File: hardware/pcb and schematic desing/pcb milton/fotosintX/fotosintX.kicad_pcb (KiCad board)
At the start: 2 copper layers, 46.5 x 74.3 mm, 12 parts, among them J4 TB_1X2, J5 TB_1X2, Q1 2N3904, U1 ESP32_DEVKITC, U2 L7805

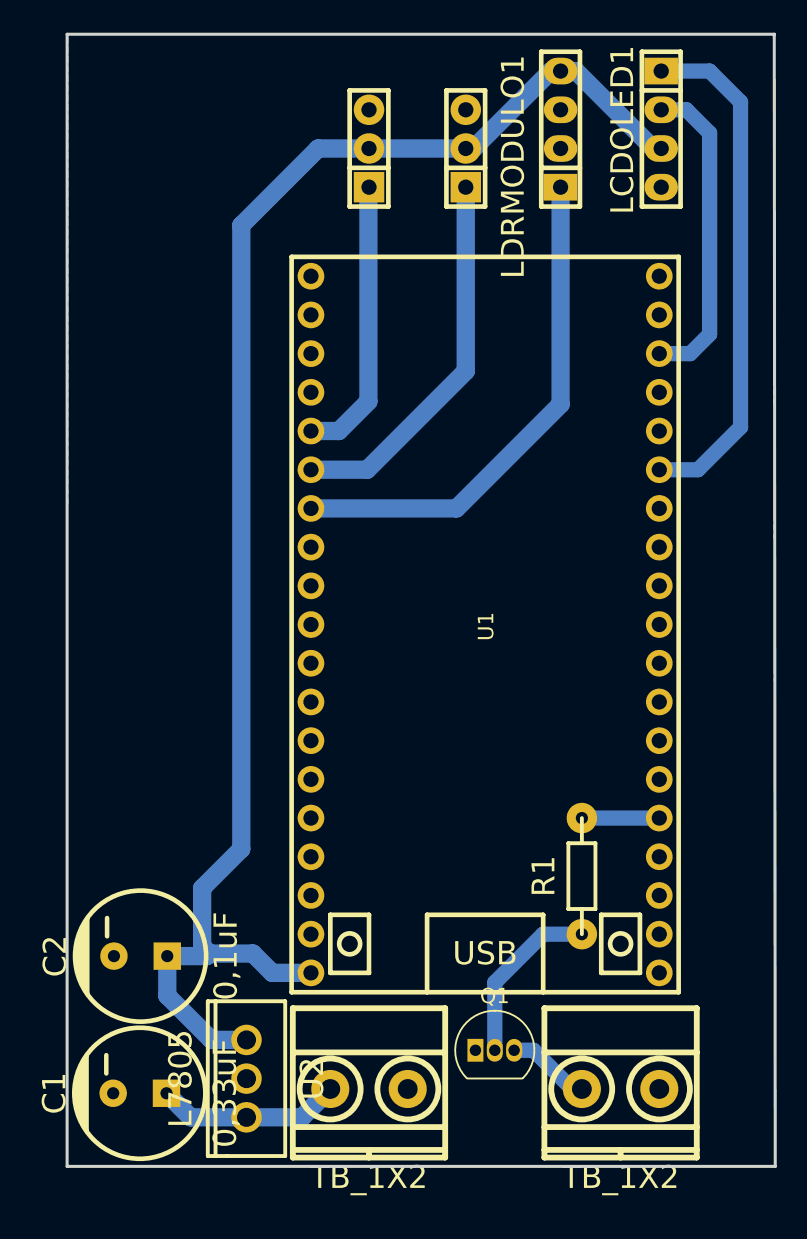
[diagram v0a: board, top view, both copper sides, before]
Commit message: Mejorando pcb
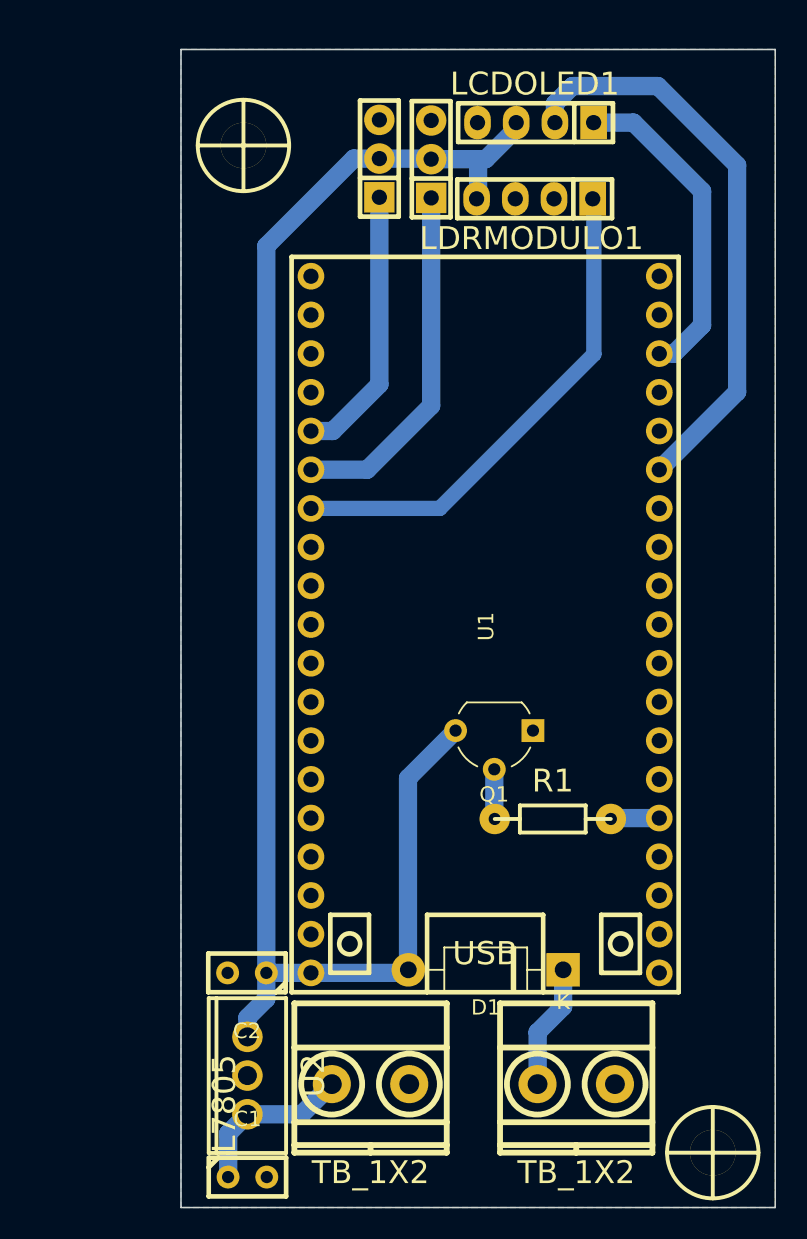
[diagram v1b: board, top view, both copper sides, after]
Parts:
- added D1: 1N4007, Diode_THT:D_DO-41_SOD81_P10.16mm_Horizontal, F.Cu at (193.1, 101.4)
- added H1: Mounting_Hole, eestn5:hole_3mm, F.Cu at (202.9, 113.4)
- added H2: Mounting_Hole, eestn5:hole_3mm, F.Cu at (172.1, 47.3)
- C1, C2: footprint eestn5:CAP_ELEC_8x11.5mm -> eestn5:CAP_0.1
- Q1: value 2N3904 -> PN2222A; footprint Package_TO_SOT_THT:TO-92_Inline -> Package_TO_SOT_THT:TO-92_Wide
- moved Q1 21.3 mm to (191.1, 85.7), turned to 180 degrees
- moved C1 8.95 mm to (172.4, 115.0), turned to 0 degrees
- moved LCDOLED1 8.26 mm to (191.3, 45.8), turned to 180 degrees
- moved C2 7.07 mm to (172.3, 101.6), turned to 180 degrees
- moved LDRMODULO1 4.88 mm to (191.2, 50.8), turned to 180 degrees
- moved R1 4.21 mm to (192.4, 91.5), turned to 0 degrees
- moved J4 2.93 mm to (193.9, 108.9)
- moved SENSORNIVELDEAGUA1 2.38 mm to (184.4, 48.2)
- moved SENSORHUMEDAD1 0.95 mm to (181.0, 48.2)
- moved J5 0.34 mm to (180.4, 108.9)
- moved U2 0.21 mm to (172.4, 108.3)
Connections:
- J4 pad 1: /motor -> +5V
- LCDOLED1 pad 1: /SDA -> /SCL
- LCDOLED1 pad 2: /SCL -> /SDA
- Q1 pad 3: /motor -> +5V
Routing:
- net Net-(Q1-B): track 11.5 -> 3.27 mm
- net +5V: track 101.9 -> 109.7 mm
- net /motor: track 5.50 -> 0.00 mm
- net /SDA: track 33.9 -> 37.9 mm
- net /ON: track 5.08 -> 3.20 mm
- net /SERIAL: track 24.9 -> 23.3 mm
- net +12V: track 12.2 -> 11.0 mm
- net /AUOT: track 18.7 -> 18.0 mm
- net /SCL: track 20.8 -> 21.4 mm
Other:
- board size 46.5 x 74.3 mm -> 39 x 76 mm
